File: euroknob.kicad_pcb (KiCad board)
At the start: 2 copper layers, 24 x 79 mm, 23 parts, among them J1 AudioJack2_SwitchT, J2 Conn_01x03_Pin, U1 CH32V003FxPx, U2 AS5600

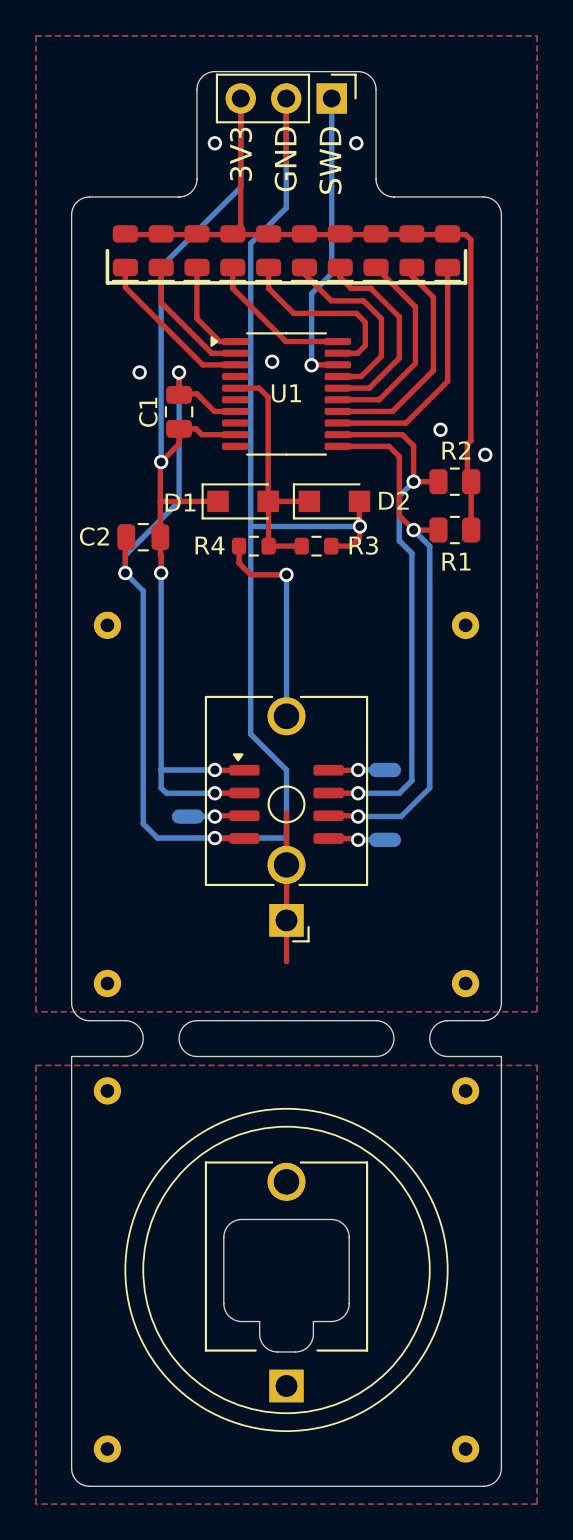
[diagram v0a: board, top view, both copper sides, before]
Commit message: rounding
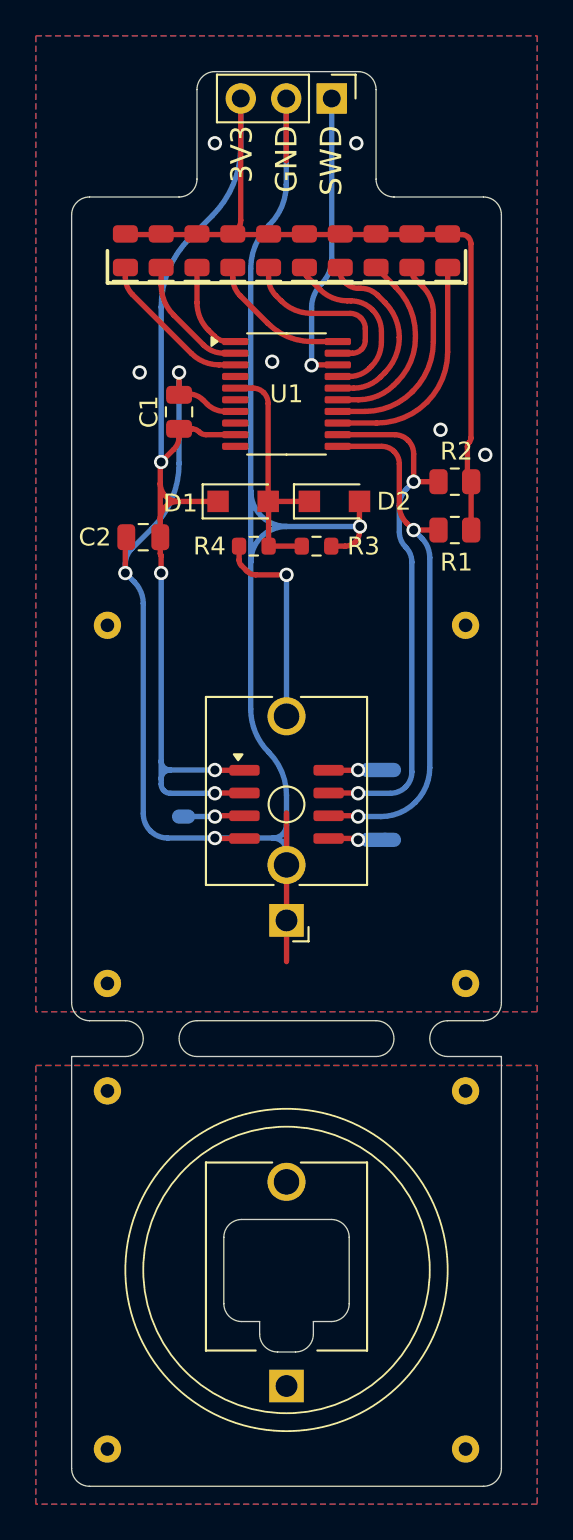
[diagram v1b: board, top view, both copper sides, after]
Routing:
- net GND: track 109.8 -> 114.1 mm
- net VCC: track 102.1 -> 104.2 mm
- net Net-(D9-K): track 11.2 -> 10.7 mm
- net /SDA: track 30.6 -> 30.1 mm
